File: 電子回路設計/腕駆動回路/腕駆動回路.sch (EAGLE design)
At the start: 38 parts, among them IC1 TC74HC244AF, U1 BTN9990LV, U2 BTN9990LV

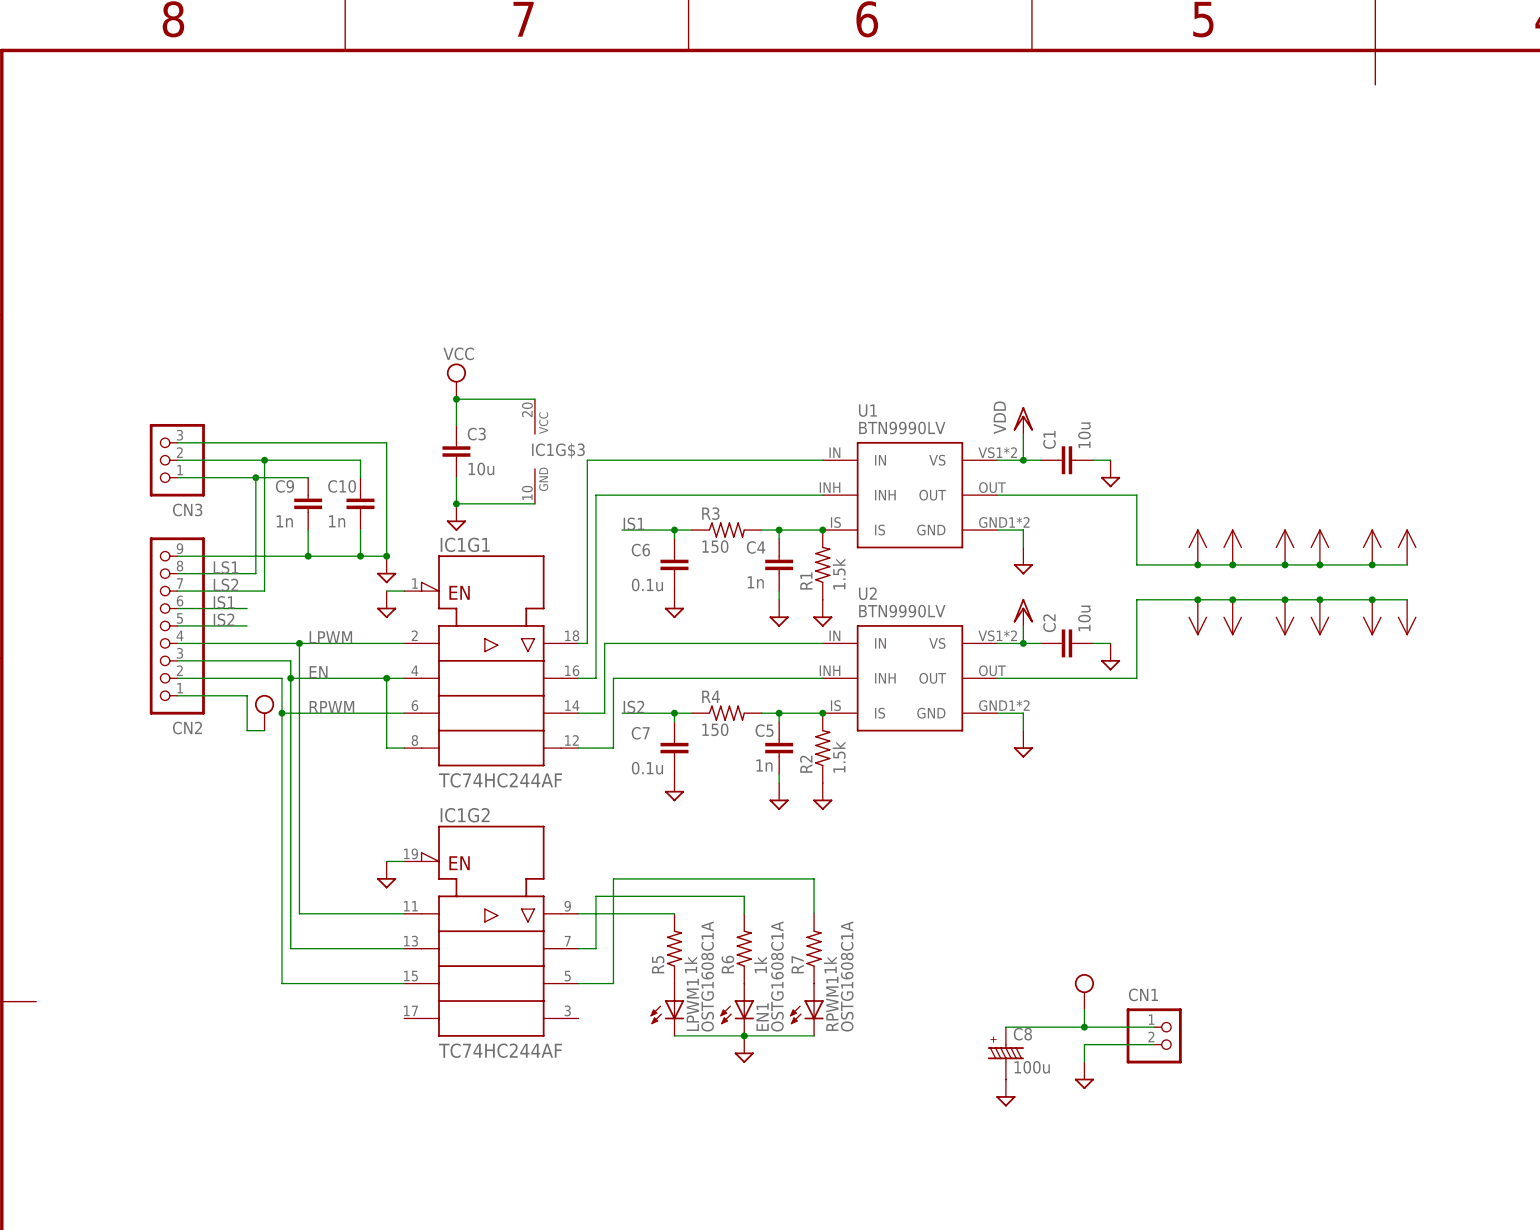
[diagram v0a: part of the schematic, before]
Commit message: add : AMD add res
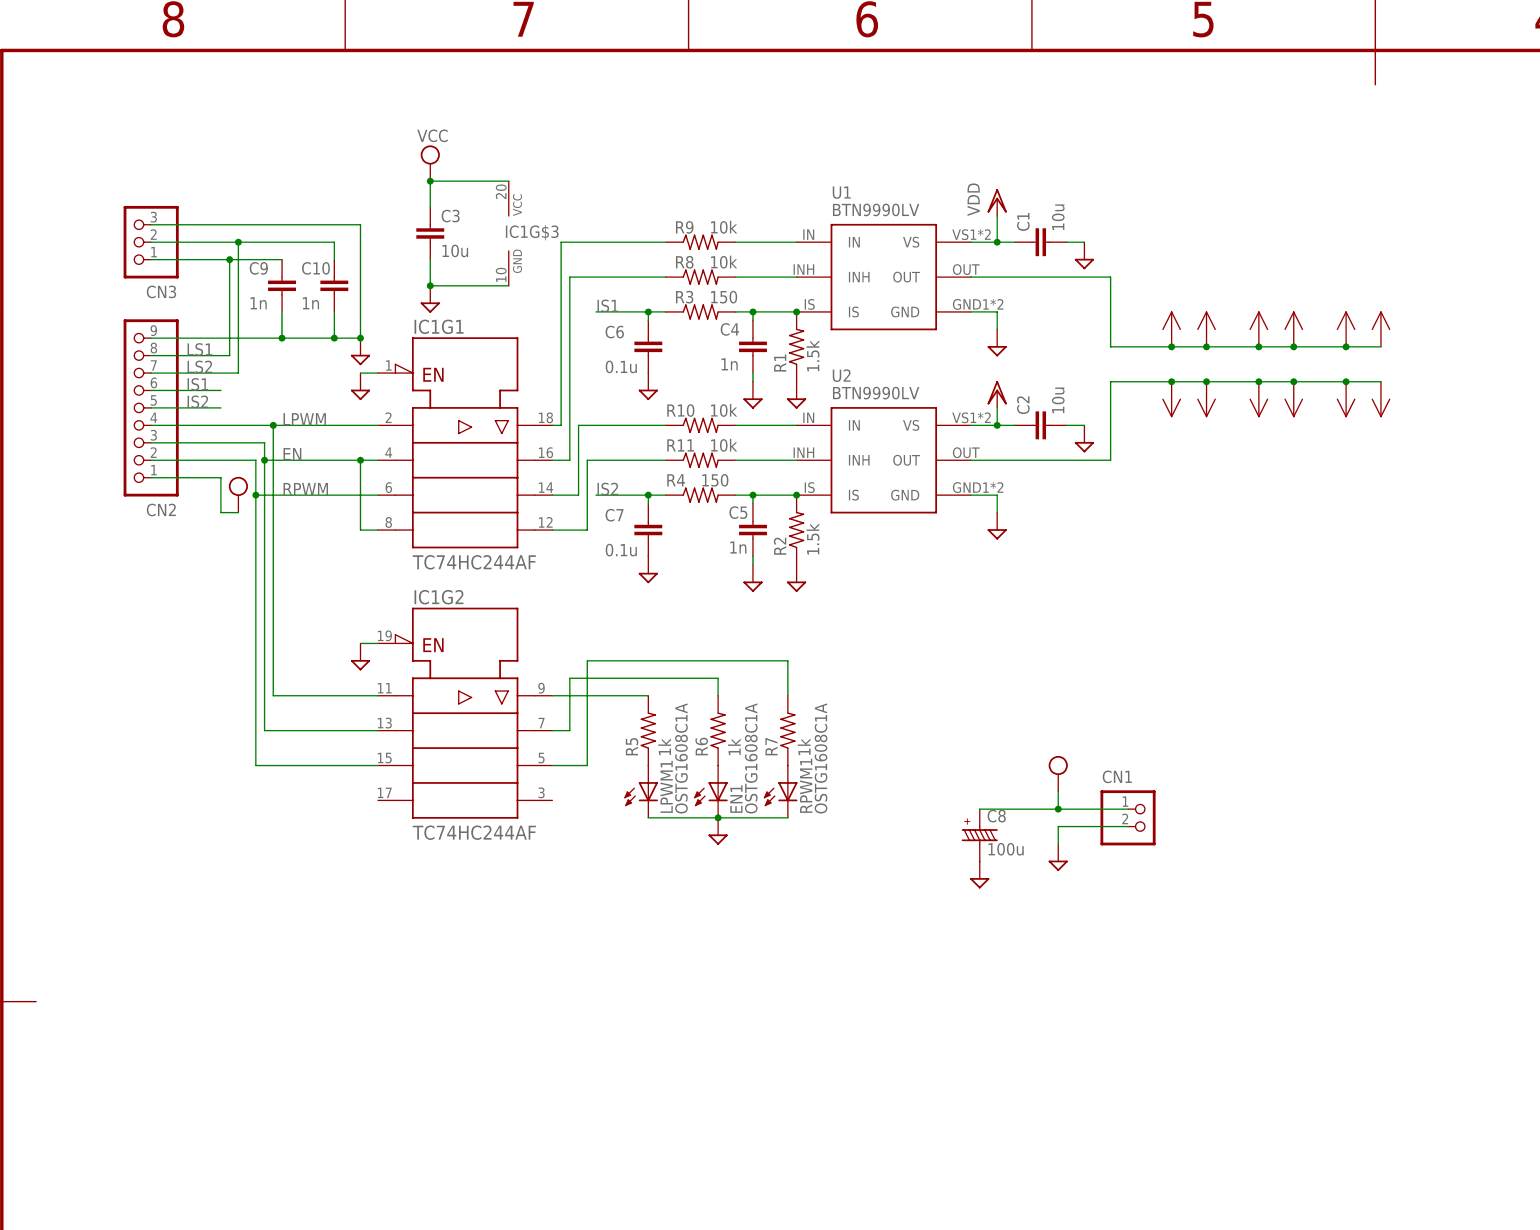
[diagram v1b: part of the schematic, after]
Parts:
- added R10, R11, R8, R9: 10k, FLE_抵抗器:RC0603J10K
- C1, C2, C3: device RCL:C2012 -> 村田製作所_チップセラミックコンデンサ:GCM31CD71H106KE36K
- C10, C4, C5, C9: device RCL:C1608 -> 村田製作所_チップセラミックコンデンサ:GCM188R91H102KA37D
- C6, C7: device RCL:C1608 -> 村田製作所_チップセラミックコンデンサ:GCM188L81H104KA57D
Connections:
- new net N$11: R8.2, U1.INH
- new net N$12: R9.2, U1.IN
- new net N$13: R10.2, U2.IN
- new net N$14: R11.2, U2.INH
- net N$1: now also R9.1; no longer U1.IN
- net N$2: now also R8.1; no longer U1.INH
- net N$3: now also R10.1; no longer U2.IN
- net N$4: now also R11.1; no longer U2.INH
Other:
- moved on the sheet: C1, C10, C2, C3, C4, C5, C6, C7, C8, C9, CN1, CN2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
